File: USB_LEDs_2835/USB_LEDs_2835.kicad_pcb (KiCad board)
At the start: 2 copper layers, 99.9 x 20 mm, 56 parts, among them U1 MT9284_1, U2 JL8022W-L, U3 74LVC1G04

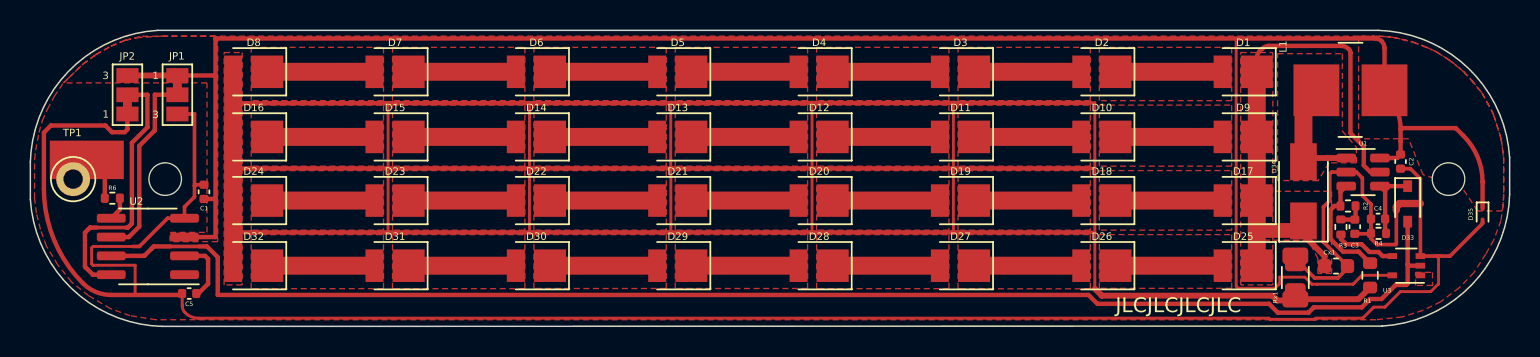
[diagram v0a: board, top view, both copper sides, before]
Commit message: Add files via upload
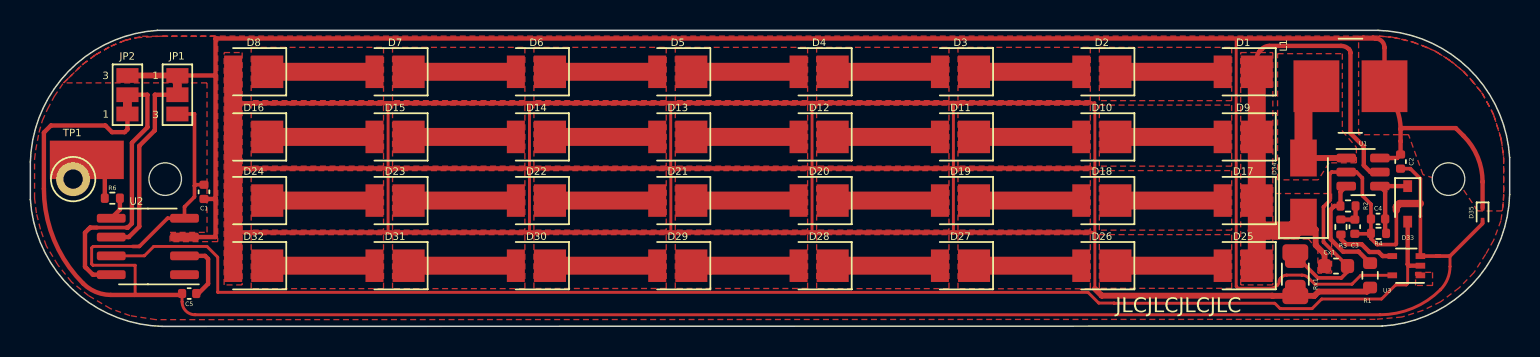
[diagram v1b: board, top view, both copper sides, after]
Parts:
- moved L1 0.27 mm to (121.8, 40.6)
- moved D34 0.25 mm to (118.7, 47.5)
- moved Rx1 0.23 mm to (118.1, 53.3)
